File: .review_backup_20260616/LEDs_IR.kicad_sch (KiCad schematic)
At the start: 13 parts, among them U30 TSOP4838

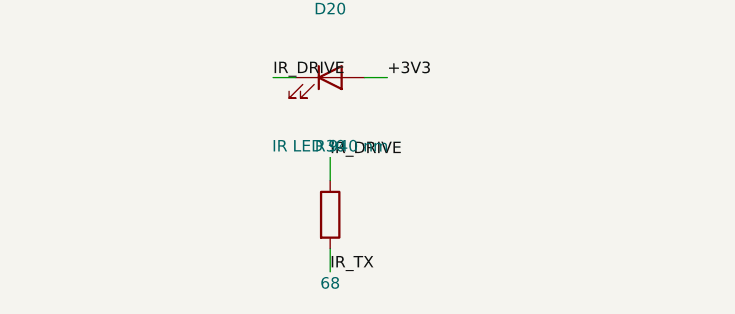
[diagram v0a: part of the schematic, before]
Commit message: checking
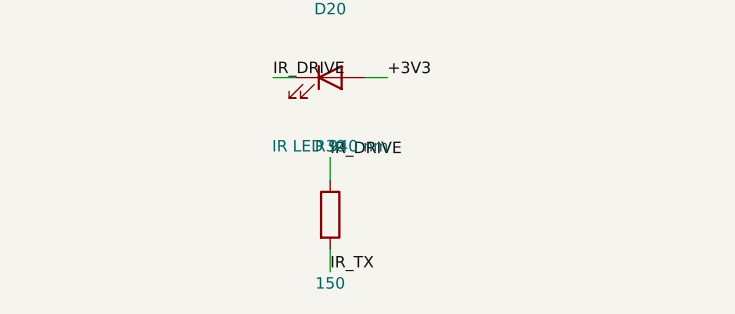
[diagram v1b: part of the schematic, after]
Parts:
- R30: value 68 -> 150
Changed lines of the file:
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@@
 		(fields_autoplaced yes)
 		(property "Reference" "R30" (at 59.69 137.16 0) (effects (font (size 1.27 1.27))))
-		(property "Value" "68" (at 59.69 152.40 0) (effects (font (size 1.27 1.27))))
+		(property "Value" "150" (at 59.69 152.40 0) (effects (font (size 1.27 1.27))))
 		(property "Footprint" "Resistor_SMD:R_0402_1005Metric" (at 59.69 144.78 0) (show_name no) (hide yes) (effects (font (size 1.27 1.27))))
 		(property "Datasheet" "" (at 59.69 144.78 0) (show_name no) (hide yes) (effects (font (size 1.27 1.27))))
